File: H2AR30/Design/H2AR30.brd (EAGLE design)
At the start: 34.6 x 30 mm, 57 parts, among them P1 HEXABIT__NO_P1_P5_P6_P7_P12, U2 INA199B2DCKT, U3 INA199B1DCKT, U4 TEXAS_INSTRUMENTS_REF2033AIDD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, X1 XTALL_CSTCE8M00G52

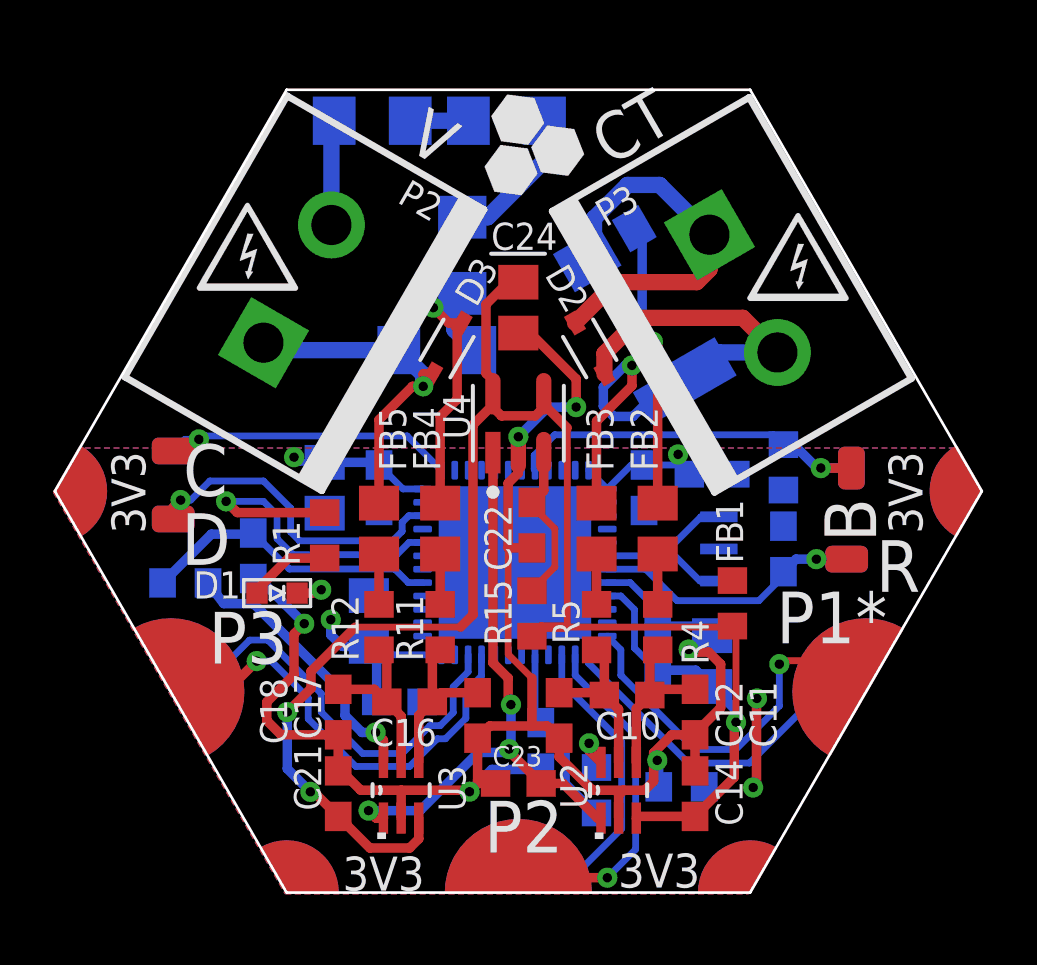
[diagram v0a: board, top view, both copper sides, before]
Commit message: final with double check
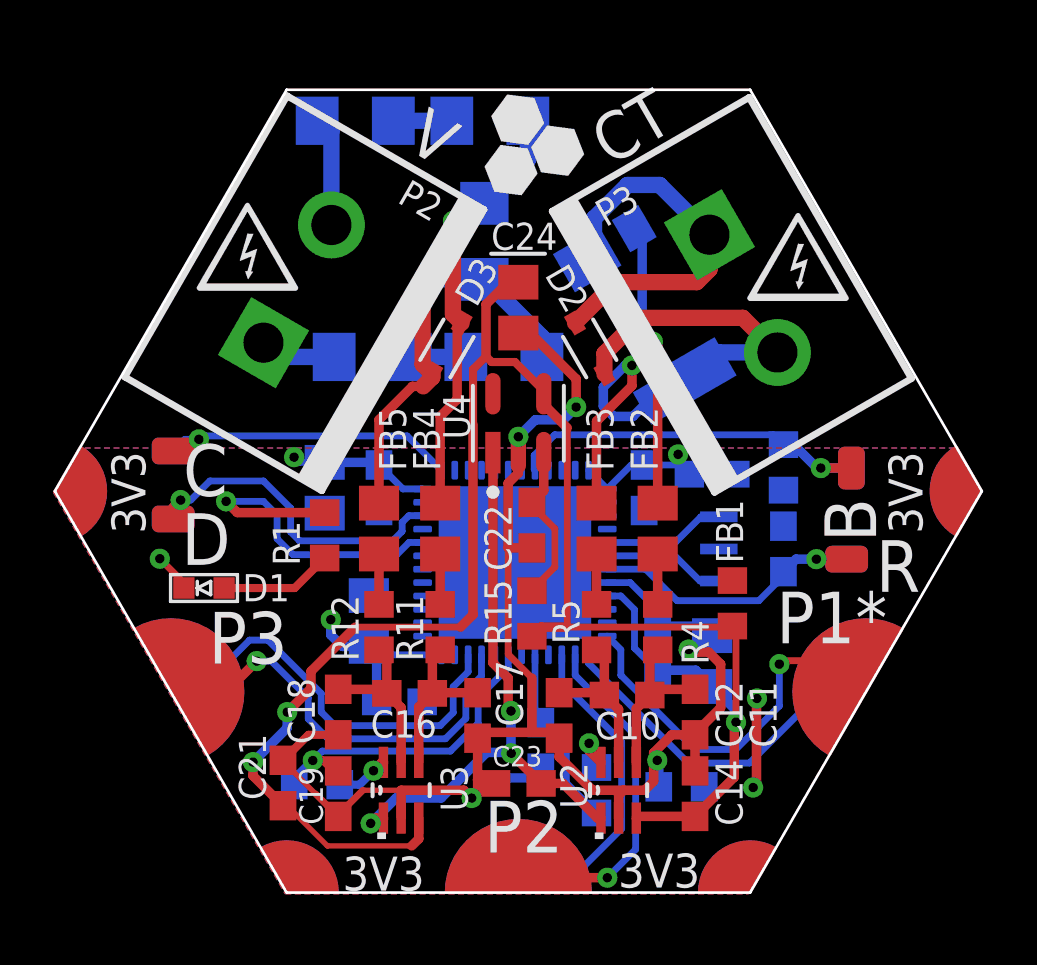
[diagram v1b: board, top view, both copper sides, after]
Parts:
- added R16: 1M0, HEXABITZ_RCLS:R1206
- moved C19 9.44 mm to (27.9, 23.4), flipped to the top
- moved R13 9.00 mm to (27.1, 23.7)
- moved R9 8.83 mm to (34.1, 39.7)
- moved R10 5.13 mm to (33.6, 48.5), turned to 0 degrees
- moved R14 4.44 mm to (33.4, 44.0), turned to 90 degrees
- moved D1 2.74 mm to (22.9, 31.1), turned to 270 degrees
- moved C21 2.10 mm to (25.9, 23.8)
- moved R8 0.64 mm to (28.6, 48.5)
- moved C16 0.32 mm to (30.6, 27.1)
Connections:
- removed net N$24: R10.2, R9.1
- removed net N$25: R8.1, R9.2
- new net N$10: R16.1, R9.2
- new net N$13: R10.2, R8.1
- new net N$22: D3.1, FB5.1, R14.1, R9.1
- new net VREF: U4.5
- net GND: now also U1.P$18
- net NEUTRAL: now also R16.2; no longer D3.1, FB5.1, R14.1
- net VCC: no longer U4.5
- net VOLTAGE_SENSE: now also U1.P$19; no longer U1.P$29
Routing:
- net N$22: track 0.00 -> 15.6 mm, vias 0 -> 1
- net NEUTRAL: track 13.0 -> 2.86 mm, vias 1 -> 0
- net N$23: track 10.3 -> 1.98 mm
- net N$24: track 5.44 -> 0.00 mm
- net AGND: track 67.4 -> 62.3 mm, vias 6 -> 5
- net N$21: track 12.7 -> 16.2 mm
- net N$5: track 2.03 -> 4.57 mm
- net N$13: track 0.00 -> 2.19 mm
- net N$25: track 2.17 -> 0.00 mm
- net N$10: track 0.00 -> 2.08 mm
- net VCC: track 69.4 -> 70.7 mm
- net N$4: track 3.14 -> 4.22 mm
- net USART3_RX: track 15.8 -> 14.9 mm
- net USART3_TX: track 16.2 -> 15.4 mm
- net VOLTAGE_SENSE: track 11.3 -> 12.1 mm, vias 0 -> 1
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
